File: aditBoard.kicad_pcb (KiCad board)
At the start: 4 copper layers, 36 parts, among them J1 USB_C_Receptacle_USB2.0, J2 Hashboard0, U2 W25X40CLUXIG TR, U3 RP2040, U4 RT9080-33GJ5, Y1 12MHz

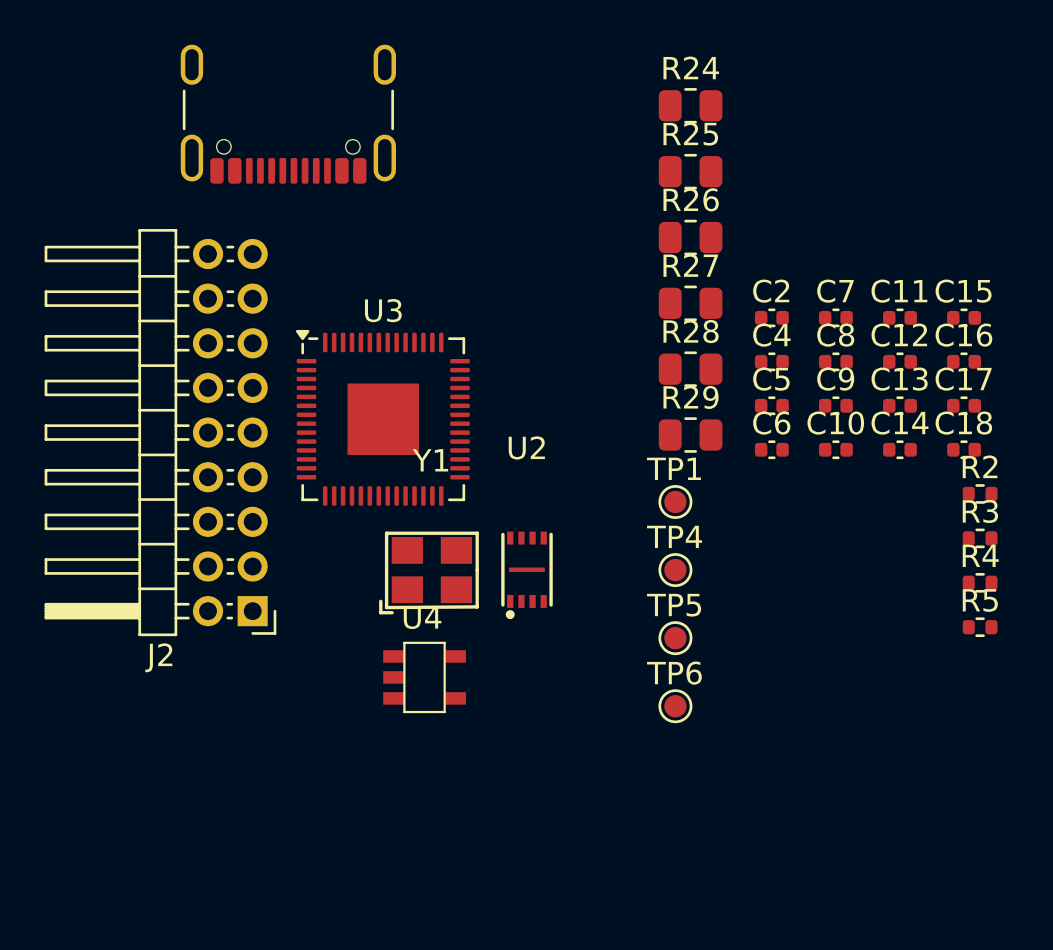
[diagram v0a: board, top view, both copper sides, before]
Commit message: pretty much routed
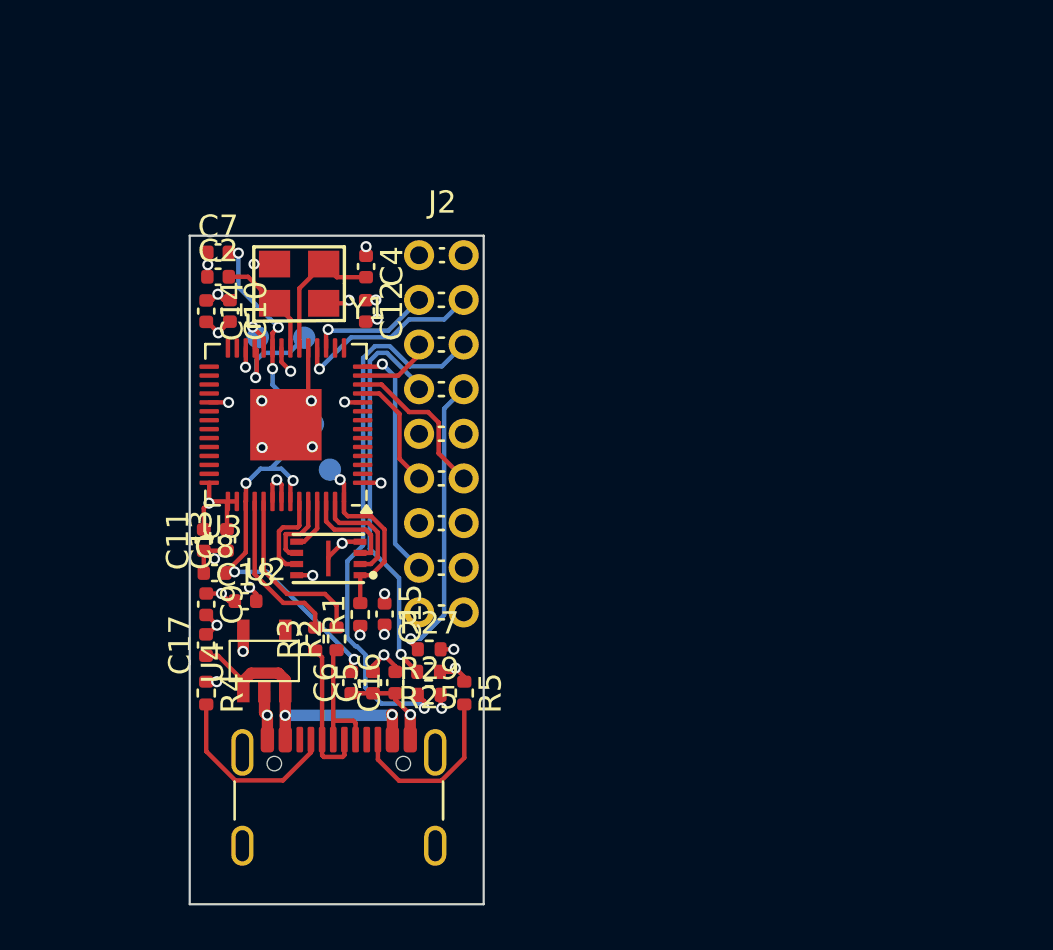
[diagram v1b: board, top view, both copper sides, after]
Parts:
- removed R24, R26, R28: 4.7K, Resistor_SMD:R_0805_2012Metric
- added R1: 10k, Resistor_SMD:R_0402_1005Metric, F.Cu at (122.0, 97.8)
- J2: footprint Connector_PinHeader_2.00mm:PinHeader_2x09_P2.00mm_Horizontal -> aditBoard:PinHeader_2x09_P2.00mm_Horizontal
- R25, R27, R29: footprint Resistor_SMD:R_0805_2012Metric -> Resistor_SMD:R_0402_1005Metric
- TP1, TP4, TP5, TP6: moved to B.Cu
- moved C17 35.6 mm to (115.1, 99.2), turned to 90 degrees
- moved R4 35.0 mm to (115.1, 101.3), turned to -90 degrees
- moved J1 32.9 mm to (121.0, 107.1), turned to 0 degrees
- moved C18 32.9 mm to (116.9, 97.2)
- moved C11 32.7 mm to (115.0, 94.5), turned to 90 degrees
- moved C14 31.7 mm to (115.1, 84.2), turned to -90 degrees
- moved C13 30.7 mm to (116.0, 94.5), turned to 90 degrees
- moved R3 30.1 mm to (120.0, 98.9), turned to 90 degrees
- moved C9 29.6 mm to (115.1, 97.4), turned to -90 degrees
- moved R2 29.6 mm to (120.9, 98.9), turned to 90 degrees
- moved C8 29.4 mm to (115.5, 96.0)
- moved C16 29.3 mm to (123.6, 100.9), turned to 90 degrees
- moved C15 29.2 mm to (123.1, 97.8), turned to -90 degrees
- moved C10 27.9 mm to (116.2, 84.2), turned to -90 degrees
- moved C7 27.8 mm to (115.6, 81.6)
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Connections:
- net /A00 renamed /A0
- net /A10 renamed /A1
- net /A20 renamed /A2
- J2 pad 11: /TXD0 -> /TXD
- J2 pad 12: /RXD0 -> /RXD
- J2 pad 15: /RST0 -> /RST
- J2 pad 3: /SDA0 -> /SDA
- J2 pad 4: /SCL0 -> /SCL
- J2 pad 5: /PLUG0 -> /PLUG
- U3 pad 11: /UART_TX -> /TXD
- U3 pad 12: /UART_RX -> /RXD
- U3 pad 13: unconnected-(U3-GPIO10-Pad13) -> /PLUG
- U3 pad 14: unconnected-(U3-GPIO11-Pad14) -> /RST
- U3 pad 17: /I2C_SDA -> /SDA
- U3 pad 18: /I2C_SCL -> /SCL
- U3 pad 8: /POWERUP -> unconnected-(U3-GPIO6-Pad8)
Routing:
- net /GND: track 0.00 -> 27.3 mm, vias 0 -> 21
- net /1V1: track 0.00 -> 27.0 mm, vias 0 -> 7
- net /A2: track 0.00 -> 24.7 mm, vias 0 -> 1
- net /3V3: track 0.00 -> 19.2 mm, vias 0 -> 15
- net /A1: track 0.00 -> 17.9 mm, vias 0 -> 1
- net /5V: track 0.00 -> 13.4 mm, vias 0 -> 2
- net /A0: track 0.00 -> 13.0 mm, vias 0 -> 1
- net /RST: track 0.00 -> 10.7 mm, vias 0 -> 1
- net /SCL: track 0.00 -> 8.73 mm, vias 0 -> 1
- net Net-(J1-CC1): track 0.00 -> 8.42 mm
- net /QSPI_SS: track 0.00 -> 8.36 mm, vias 0 -> 1
- net Net-(U3-USB_DP): track 0.00 -> 8.00 mm
- net Net-(J1-CC2): track 0.00 -> 7.98 mm
- net Net-(U3-USB_DM): track 0.00 -> 7.33 mm
- net /RXD: track 0.00 -> 7.08 mm
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- added copper zone on In2.Cu, net /3V3
- added copper zone on In1.Cu, net /GND
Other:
- board outline added: 13.2 x 30 mm
